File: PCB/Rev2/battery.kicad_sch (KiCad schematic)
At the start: 6 parts

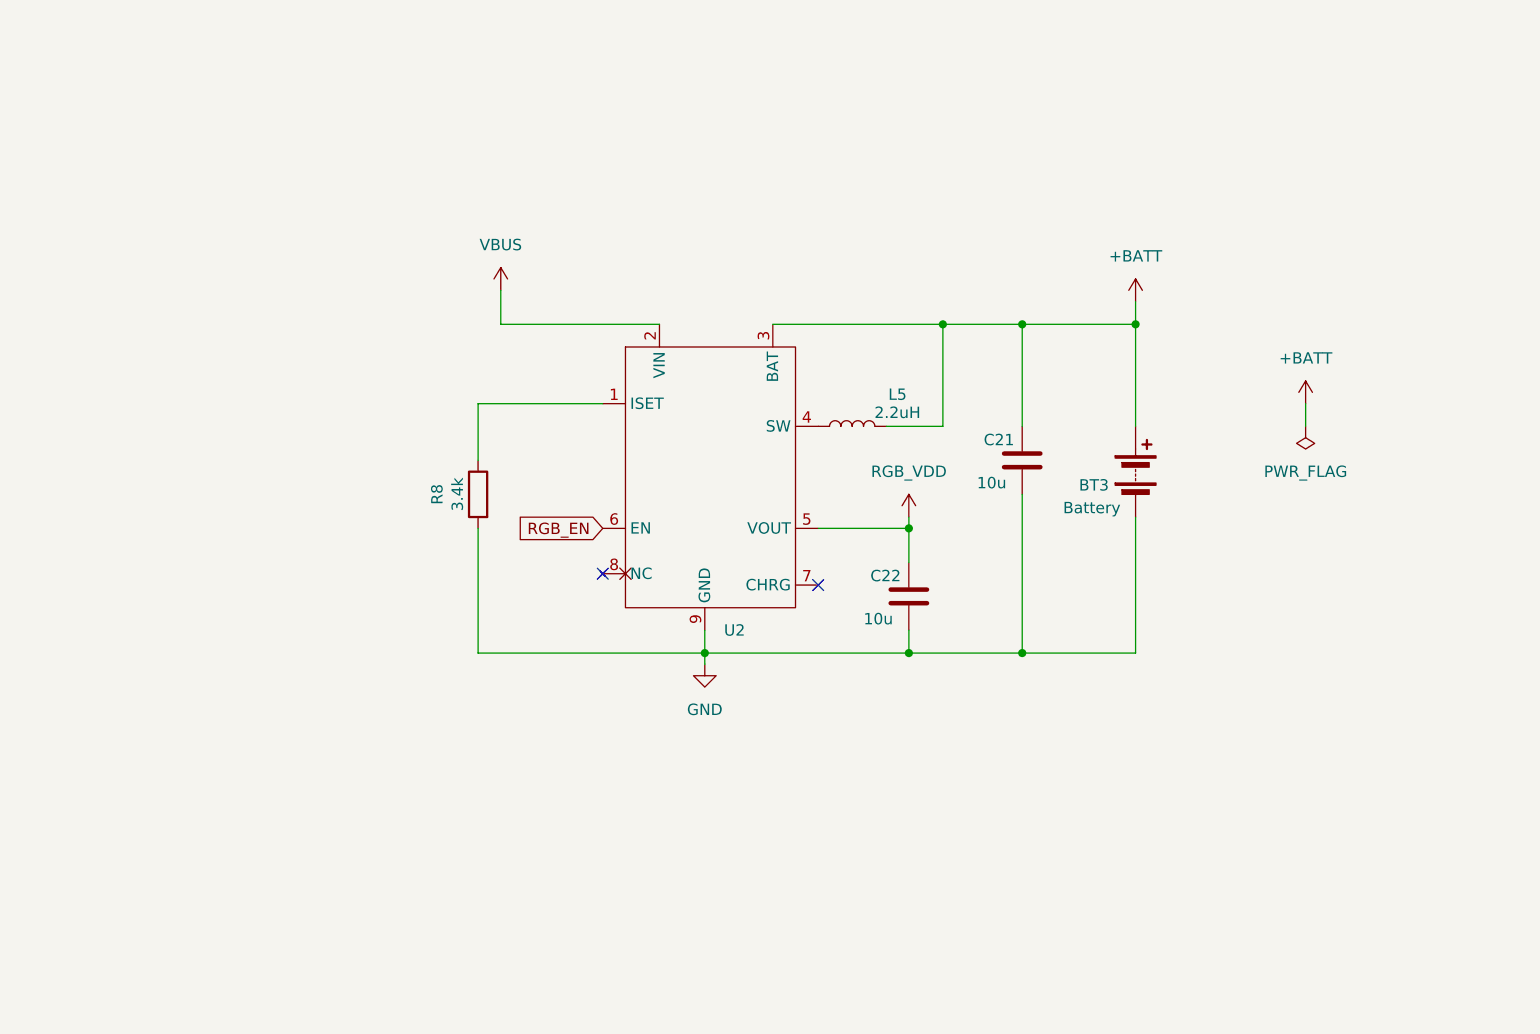
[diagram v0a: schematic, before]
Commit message: 电源芯片设计
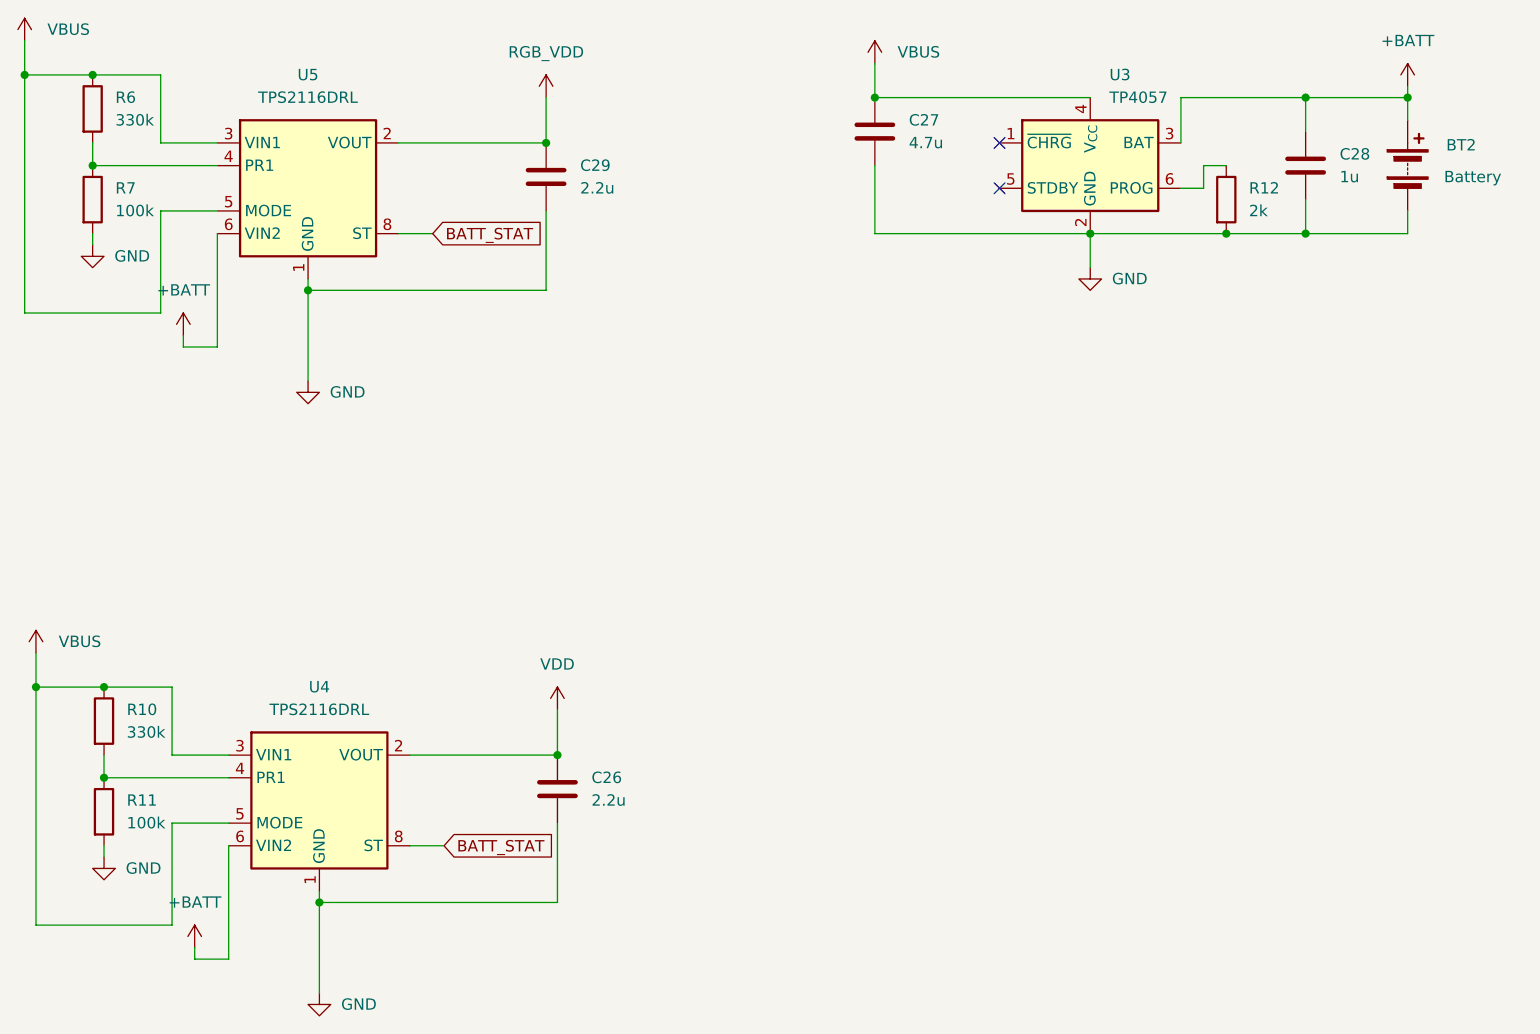
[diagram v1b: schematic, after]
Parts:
- removed BT3: Battery, Connector_Molex:Molex_Panelmate_53780-0270_1x02-1MP_P1.25mm_Horizontal, symbol Device:Battery
- removed C21, C22: 10u, Capacitor_SMD:C_0402_1005Metric, symbol Device:C
- removed L5: 2.2uH, Inductor_SMD:L_Changjiang_FNR252012S, symbol Device:L
- removed R8: 3.4k, PCM_Resistor_SMD_AKL:R_0402_1005Metric, symbol Device:R
- removed U2: ~, Package_SO:SOIC-8-1EP_3.9x4.9mm_P1.27mm_EP2.41x3.3mm, symbol LP7801D_sym:LP7801D
- added BT2: Battery, Connector_Molex:Molex_PicoBlade_53261-0271_1x02-1MP_P1.25mm_Horizontal, symbol Device:Battery
- added C26, C29: 2.2u, Capacitor_SMD:C_0402_1005Metric, symbol Device:C
- added C27: 4.7u, Capacitor_SMD:C_0402_1005Metric, symbol Device:C
- added C28: 1u, Capacitor_SMD:C_0402_1005Metric, symbol Device:C
- added R10, R6: 330k, Resistor_SMD:R_0402_1005Metric, symbol Device:R
- added R11, R7: 100k, Resistor_SMD:R_0402_1005Metric, symbol Device:R
- added R12: 2k, Resistor_SMD:R_0402_1005Metric, symbol Device:R
- added U3: TP4057, Package_TO_SOT_SMD:TSOT-23-6, symbol Battery_Management:TP4057
- added U4, U5: TPS2116DRL, Package_TO_SOT_SMD:SOT-583-8, symbol Power_Management:TPS2116DRL
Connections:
- net +BATT: now also BT2.1 (+), C28.1, U3.3 (BAT), U4.6 (VIN2), U5.6 (VIN2)
- net GND: now also BT2.2 (-), C26.2, C27.2, C28.2, C29.2, R11.2, R12.2, R7.2, U3.2 (GND), U4.1 (GND), U5.1 (GND)
- net RGB_VDD: now also C29.1, U5.2 (VOUT), U5.7 (VOUT)
- net VBUS: now also C27.1, R10.1, R6.1, U3.4 (V_{CC}), U4.3 (VIN1), U4.5 (MODE), U5.3 (VIN1), U5.5 (MODE)
- new net: R10.2, R11.1, U4.4 (PR1)
- new net: R6.2, R7.1, U5.4 (PR1)
- new net: R12.1, U3.6 (PROG)
- new net BATT_STAT: U4.8 (ST), U5.8 (ST)
- new net VDD: C26.1, U4.2 (VOUT), U4.7 (VOUT)
